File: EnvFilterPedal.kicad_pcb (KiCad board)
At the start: 4 copper layers, 80 x 52 mm, 114 parts, among them J101 ScopeGroundLoop, J102 IO, Q101 BC857, Q102 BC857, Q103 BC847, U101 TL074, U102 TL074, U103 TL074, U104 LM13700, U105 AZ34063U

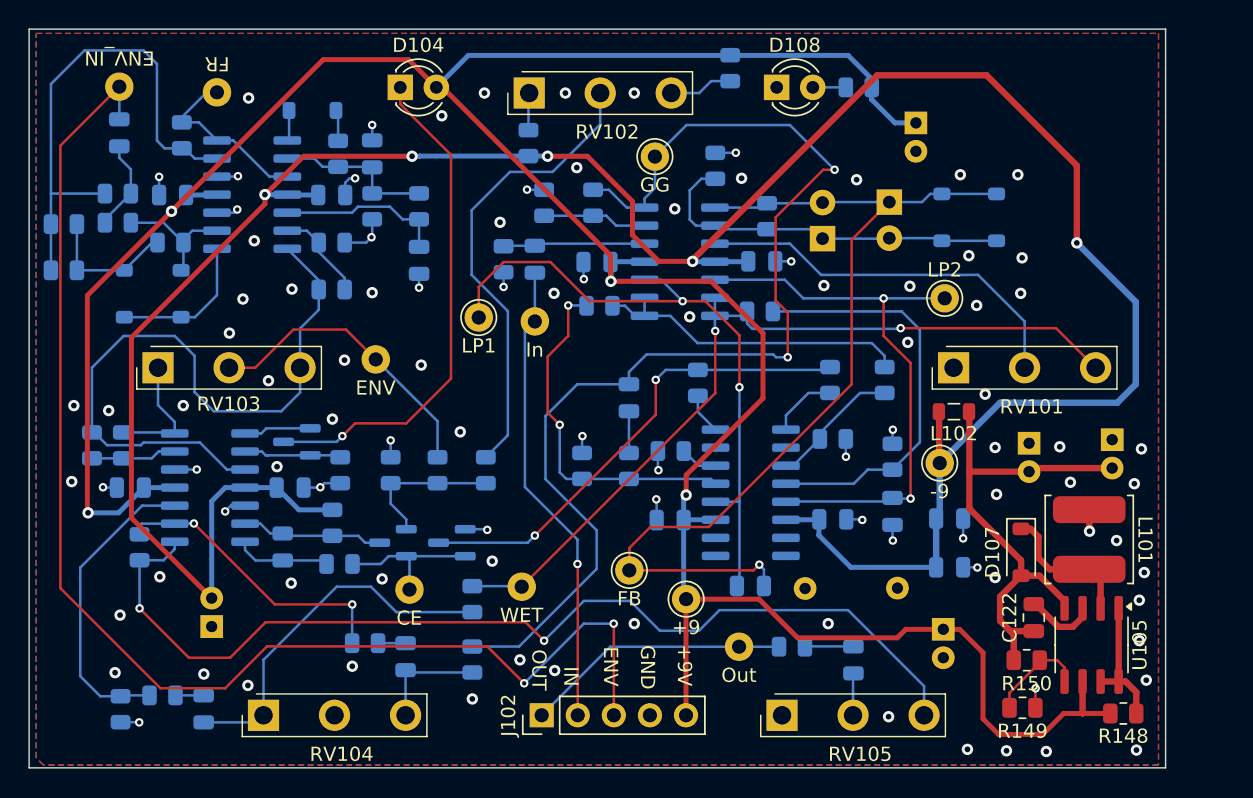
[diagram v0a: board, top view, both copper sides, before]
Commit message: new layout
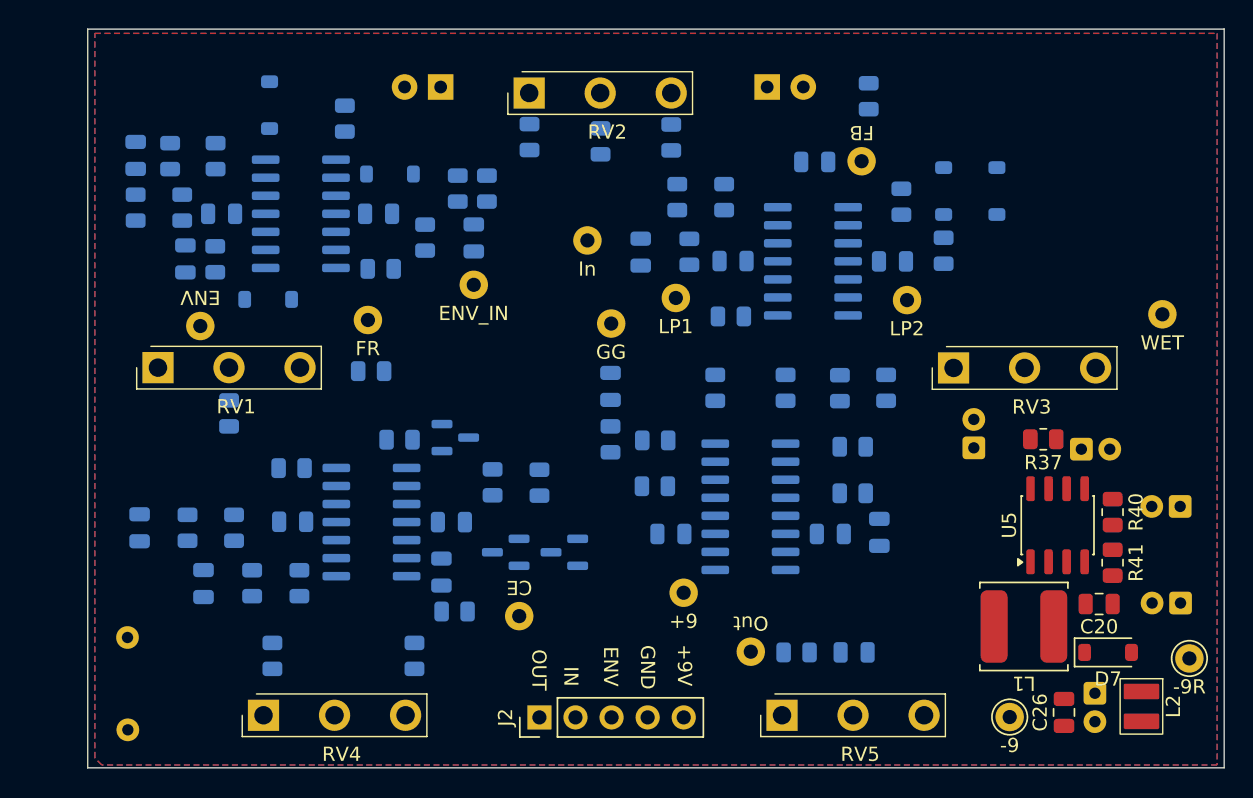
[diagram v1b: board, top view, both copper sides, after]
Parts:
- removed C101, C102, C103, C106, C108, C111, C112, C114, C115, C126: 100n, Capacitor_SMD:C_0805_2012Metric
- removed C104, C109, C113, C118, C119, C120, C125: 1u, Capacitor_SMD:C_0805_2012Metric
- removed C105: 220u, Capacitor_THT:CP_Radial_D5.0mm_P2.00mm
- removed C107: 4n7, Capacitor_SMD:C_0805_2012Metric
- removed C110: 33n, Capacitor_SMD:C_0805_2012Metric
- removed C116, C117: 1n, Capacitor_SMD:C_0805_2012Metric
- removed C121: 100u, Capacitor_THT:CP_Radial_D5.0mm_P2.00mm
- removed C122: 470p, Capacitor_SMD:C_0805_2012Metric
- removed C123, C124: 470u, Capacitor_THT:CP_Radial_D5.0mm_P2.00mm
- removed D101, D102, D103, D109, D110: 1N4148W, Diode_SMD:D_SOD-123
- removed D104, D105, D106, D108: LED, LED_THT:LED_D3.0mm
- removed D107: PMEG3030, Diode_SMD:D_SOD-123
- removed J101: ScopeGroundLoop, Connector:THT_GND_WIRE
- removed J102: IO, Connector_PinHeader_2.54mm:PinHeader_1x05_P2.54mm_Vertical
- removed L101: 68uH, Inductor_SMD:L_TDK_VLS6045EX_VLS6045AF
- removed L102: 1u, Inductor_SMD:L_0805_2012Metric
- removed Q101, Q102: BC857, Package_TO_SOT_SMD:SOT-23
- removed Q103: BC847, Package_TO_SOT_SMD:SOT-23
- removed R101, R102, R103, R104, R105, R108, R112, R113, R117, R118, R120, R124: 100k, Resistor_SMD:R_0805_2012Metric
- removed R106, R125, R126, R129, R130: 1k, Resistor_SMD:R_0805_2012Metric
- removed R107: 22k, Resistor_SMD:R_0805_2012Metric
- removed R109: 5k1, Resistor_SMD:R_0805_2012Metric
- removed R110, R136: 6k8, Resistor_SMD:R_0805_2012Metric
- removed R111, R135: 10k, Resistor_SMD:R_0805_2012Metric
- removed R114, R119: 2k2, Resistor_SMD:R_0805_2012Metric
- removed R115, R137, R139: 470k, Resistor_SMD:R_0805_2012Metric
- removed R116, R133, R134: 4k7, Resistor_SMD:R_0805_2012Metric
- removed R121: 1M, Resistor_SMD:R_0805_2012Metric
- removed R122, R141, R142: 47k, Resistor_SMD:R_0805_2012Metric
- removed R123, R154: 12k, Resistor_SMD:R_0805_2012Metric
- removed R127, R128, R131, R132: 33k, Resistor_SMD:R_0805_2012Metric
- removed R138, R140: 1Meg, Resistor_SMD:R_0805_2012Metric
- removed R143: 220, Resistor_SMD:R_0805_2012Metric
- removed R148: 0.24R, Resistor_SMD:R_0805_2012Metric
- removed R149: 51k, Resistor_SMD:R_0805_2012Metric
- removed R150: 8k2, Resistor_SMD:R_0805_2012Metric
- removed RV101, RV104: 100kB, Potentiometer_THT:Potentiometer_Alpha_RV16AF_42_VeryLong
- removed RV102, RV103: 10kB, Potentiometer_THT:Potentiometer_Alpha_RV16AF_42_VeryLong
- removed RV105: 100kA, Potentiometer_THT:Potentiometer_Alpha_RV16AF_42_VeryLong
- removed TP101: In, TestPoint:TestPoint_THTPad_D2.0mm_Drill1.0mm_VAL
- removed TP102: Out, TestPoint:TestPoint_THTPad_D2.0mm_Drill1.0mm_VAL
- removed TP103: CE, TestPoint:TestPoint_THTPad_D2.0mm_Drill1.0mm_VAL
- removed TP104: WET, TestPoint:TestPoint_THTPad_D2.0mm_Drill1.0mm_VAL
- removed TP105: ENV, TestPoint:TestPoint_THTPad_D2.0mm_Drill1.0mm_VAL
- removed TP106: ENV_IN, TestPoint:TestPoint_THTPad_D2.0mm_Drill1.0mm_VAL
- removed TP107: GG, TestPoint:TestPoint_THTPad_D2.0mm_Drill1.0mm_VAL
- removed TP108: FR, TestPoint:TestPoint_THTPad_D2.0mm_Drill1.0mm_VAL
- removed TP109: +9, TestPoint:TestPoint_THTPad_D2.0mm_Drill1.0mm_VAL
- removed TP110: -9, TestPoint:TestPoint_THTPad_D2.0mm_Drill1.0mm_VAL
- removed TP111: LP1, TestPoint:TestPoint_THTPad_D2.0mm_Drill1.0mm_VAL
- removed TP112: LP2, TestPoint:TestPoint_THTPad_D2.0mm_Drill1.0mm_VAL
- removed TP113: FB, TestPoint:TestPoint_THTPad_D2.0mm_Drill1.0mm_VAL
- removed U101, U102, U103: TL074, Package_SO:SOIC-14_3.9x8.7mm_P1.27mm
- removed U104: LM13700, Package_SO:SOIC-16_3.9x9.9mm_P1.27mm
- removed U105: AZ34063U, Package_SO:SO-8_3.9x4.9mm_P1.27mm
- added C10: 100n, Capacitor_SMD:C_0805_2012Metric, B.Cu at (60.4, 80.2)
- added C11: 1u, Capacitor_SMD:C_0805_2012Metric, B.Cu at (15.0, 60.9)
- added C12: 1u, Capacitor_SMD:C_0805_2012Metric, B.Cu at (44.9, 69.8)
- added C13: 33n, Capacitor_SMD:C_0805_2012Metric, B.Cu at (11.5, 53.6)
- added C14: 1n, Capacitor_SMD:C_0805_2012Metric, B.Cu at (59.3, 54.0)
- added C15: 1n, Capacitor_SMD:C_0805_2012Metric, B.Cu at (63.9, 80.1)
- added C16: 4n7, Capacitor_SMD:C_0805_2012Metric, B.Cu at (33.0, 82.9)
- added C17: 220u, Capacitor_THT:CP_Radial_D5.0mm_P2.00mm, B.Cu at (78.1, 74.3)
- added C18: 1u, Capacitor_SMD:C_0805_2012Metric, B.Cu at (16.3, 83.7)
- added C19: 1u, Capacitor_SMD:C_0805_2012Metric, B.Cu at (11.8, 79.8)
- added C2: 100n, Capacitor_SMD:C_0805_2012Metric, B.Cu at (17.6, 57.7)
- added C20: 470p, Capacitor_SMD:C_0805_2012Metric, F.Cu at (79.3, 85.2)
- added C21: 220u, Capacitor_THT:CP_Radial_D5.0mm_P2.00mm, B.Cu at (85.1, 85.1)
- added C22: 470u, Capacitor_THT:CP_Radial_D5.0mm_P2.00mm, B.Cu at (85.0, 78.3)
- added C23: 1u, Capacitor_SMD:C_0805_2012Metric, B.Cu at (62.1, 88.6)
- added C24: 220u, Capacitor_THT:CP_Radial_D5.0mm_P2.00mm, B.Cu at (79.0, 91.4)
- added C25: 100u, Capacitor_THT:CP_Radial_D5.0mm_P2.00mm, B.Cu at (70.5, 74.2)
- added C26: 10u, Capacitor_SMD:C_0805_2012Metric, F.Cu at (76.8, 92.8)
- added C3: 100n, Capacitor_SMD:C_0805_2012Metric, B.Cu at (22.6, 79.4)
- added C4: 100n, Capacitor_SMD:C_0805_2012Metric, B.Cu at (33.7, 79.4)
- added C5: 100n, Capacitor_SMD:C_0805_2012Metric, B.Cu at (35.3, 59.4)
- added C6: 1u, Capacitor_SMD:C_0805_2012Metric, B.Cu at (47.0, 60.4)
- added C7: 100n, Capacitor_SMD:C_0805_2012Metric, B.Cu at (53.5, 61.0)
- added C8: 100n, Capacitor_SMD:C_0805_2012Metric, B.Cu at (64.8, 61.0)
- added C9: 100n, Capacitor_SMD:C_0805_2012Metric, B.Cu at (49.2, 80.2)
- added D1: 1N4148W, Diode_SMD:D_SOD-123, B.Cu at (29.4, 54.9)
- added D2: 1N4148W, Diode_SMD:D_SOD-123, B.Cu at (20.9, 50.0)
- added D3: 1N4148W, Diode_SMD:D_SOD-123, B.Cu at (20.8, 63.7)
- added D4: 1N4148W, Diode_SMD:D_SOD-123, B.Cu at (68.4, 56.1)
- added D5: 1N4148W, Diode_SMD:D_SOD-123, B.Cu at (72.1, 56.1)
- added D6: LED, LED_THT:LED_D3.0mm, B.Cu at (33.0, 48.8)
- added D7: PMEG3030, Diode_SMD:D_SOD-123, F.Cu at (80.0, 88.6)
- added D8: LED, LED_THT:LED_D3.0mm, B.Cu at (56.0, 48.8)
- added J1: ScopeGroundLoop, Connector_Pin:THT_GND_WIRE, B.Cu at (10.9, 90.6)
- added J2: IO, Connector_PinHeader_2.54mm:PinHeader_1x05_P2.54mm_Vertical, F.Cu at (39.9, 93.2)
- added L1: 68uH, Inductor_SMD:L_TDK_VLS6045EX_VLS6045AF, F.Cu at (74.0, 86.8)
- added L2: 4u7, Inductor_SMD:L_Bourns_SRP3212, F.Cu at (82.3, 92.4)
- added Q1: BC847, Package_TO_SOT_SMD:SOT-23, B.Cu at (34.0, 73.5)
- added Q2: BC857, Package_TO_SOT_SMD:SOT-23, B.Cu at (37.5, 81.5)
- added Q3: BC857, Package_TO_SOT_SMD:SOT-23, B.Cu at (41.7, 81.5)
- added R1: 100k, Resistor_SMD:R_0805_2012Metric, B.Cu at (36.2, 55.9)
- added R10: 47k, Resistor_SMD:R_0805_2012Metric, B.Cu at (34.2, 55.9)
- added R11: 100k, Resistor_SMD:R_0805_2012Metric, B.Cu at (31.9, 59.4)
- added R12: 22k, Resistor_SMD:R_0805_2012Metric, B.Cu at (14.8, 57.3)
- added R13: 33k, Resistor_SMD:R_0805_2012Metric, B.Cu at (44.9, 73.6)
- added R14: 100k, Resistor_SMD:R_0805_2012Metric, B.Cu at (28.8, 61.6)
- added R15: 1k, Resistor_SMD:R_0805_2012Metric, B.Cu at (48.0, 76.9)
- added R16: 100k, Resistor_SMD:R_0805_2012Metric, B.Cu at (11.5, 57.3)
- added R17: 1k, Resistor_SMD:R_0805_2012Metric, B.Cu at (48.1, 73.7)
- added R18: 33k, Resistor_SMD:R_0805_2012Metric, B.Cu at (53.4, 64.9)
- added R19: 4k7, Resistor_SMD:R_0805_2012Metric, B.Cu at (52.3, 70.0)
- added R2: 1M, Resistor_SMD:R_0805_2012Metric, B.Cu at (50.5, 60.4)
- added R20: 5k1, Resistor_SMD:R_0805_2012Metric, B.Cu at (13.9, 53.6)
- added R21: 100k, Resistor_SMD:R_0805_2012Metric, B.Cu at (17.1, 53.6)
- added R22: 10k, Resistor_SMD:R_0805_2012Metric, B.Cu at (65.4, 56.9)
- added R23: 33k, Resistor_SMD:R_0805_2012Metric, B.Cu at (61.1, 70.0)
- added R24: 1k, Resistor_SMD:R_0805_2012Metric, B.Cu at (62.0, 77.4)
- added R25: 2k2, Resistor_SMD:R_0805_2012Metric, B.Cu at (30.1, 73.6)
- added R26: 6k8, Resistor_SMD:R_0805_2012Metric, B.Cu at (68.4, 60.3)
- added R27: 1k, Resistor_SMD:R_0805_2012Metric, B.Cu at (62.0, 74.1)
- added R28: 33k, Resistor_SMD:R_0805_2012Metric, B.Cu at (64.3, 70.0)
- added R29: 4k7, Resistor_SMD:R_0805_2012Metric, B.Cu at (57.2, 70.0)
- added R3: 100k, Resistor_SMD:R_0805_2012Metric, B.Cu at (28.1, 68.8)
- added R30: 6k8, Resistor_SMD:R_0805_2012Metric, B.Cu at (49.2, 52.3)
- added R31: 10k, Resistor_SMD:R_0805_2012Metric, B.Cu at (39.2, 52.3)
- added R32: 100k, Resistor_SMD:R_0805_2012Metric, B.Cu at (18.1, 71.8)
- added R33: 100k, Resistor_SMD:R_0805_2012Metric, B.Cu at (44.2, 52.6)
- added R34: 2k2, Resistor_SMD:R_0805_2012Metric, B.Cu at (39.9, 76.6)
- added R35: 470k, Resistor_SMD:R_0805_2012Metric, B.Cu at (36.6, 76.6)
- added R36: 4k7, Resistor_SMD:R_0805_2012Metric, B.Cu at (34.0, 85.7)
- added R37: 0.24R, Resistor_SMD:R_0805_2012Metric, F.Cu at (75.4, 73.6)
- added R38: 47k, Resistor_SMD:R_0805_2012Metric, B.Cu at (21.1, 88.8)
- added R39: 47k, Resistor_SMD:R_0805_2012Metric, B.Cu at (31.1, 88.8)
- added R4: 12k, Resistor_SMD:R_0805_2012Metric, B.Cu at (49.6, 56.5)
- added R40: 51k, Resistor_SMD:R_0805_2012Metric, F.Cu at (80.3, 78.7)
- added R41: 8k2, Resistor_SMD:R_0805_2012Metric, F.Cu at (80.3, 82.3)
- added R42: 470k, Resistor_SMD:R_0805_2012Metric, B.Cu at (19.7, 83.7)
- added R43: 470k, Resistor_SMD:R_0805_2012Metric, B.Cu at (15.2, 79.8)
- added R44: 1Meg, Resistor_SMD:R_0805_2012Metric, B.Cu at (18.4, 79.8)
- added R45: 1Meg, Resistor_SMD:R_0805_2012Metric, B.Cu at (23.0, 83.7)
- added R46: 220, Resistor_SMD:R_0805_2012Metric, B.Cu at (58.0, 88.6)
- added R47: 12k, Resistor_SMD:R_0805_2012Metric, B.Cu at (63.1, 49.4)
- added R5: 100k, Resistor_SMD:R_0805_2012Metric, B.Cu at (26.2, 51.0)
- added R6: 47k, Resistor_SMD:R_0805_2012Metric, B.Cu at (52.9, 56.5)
- added R7: 100k, Resistor_SMD:R_0805_2012Metric, B.Cu at (22.5, 75.6)
- added R8: 1k, Resistor_SMD:R_0805_2012Metric, B.Cu at (17.1, 60.9)
- added RV1: 10kB, Potentiometer_THT:Potentiometer_Alpha_RV16AF_42_Single_Long, F.Cu at (13.1, 68.5)
- added RV2: 10kB, Potentiometer_THT:Potentiometer_Alpha_RV16AF_42_Single_Long, F.Cu at (39.2, 49.2)
- added RV3: 100kB, Potentiometer_THT:Potentiometer_Alpha_RV16AF_42_Single_Long, F.Cu at (69.1, 68.5)
- added RV4: 100kB, Potentiometer_THT:Potentiometer_Alpha_RV16AF_42_Single_Long, F.Cu at (20.5, 93.0)
- added RV5: 100kA, Potentiometer_THT:Potentiometer_Alpha_RV16AF_42_Single_Long, F.Cu at (57.0, 93.0)
- added TP1: LP1, TestPoint:TestPoint_THTPad_D2.0mm_Drill1.0mm_VAL, B.Cu at (49.5, 63.6)
- added TP10: ENV, TestPoint:TestPoint_THTPad_D2.0mm_Drill1.0mm_VAL, B.Cu at (16.1, 65.6)
- added TP11: ENV_IN, TestPoint:TestPoint_THTPad_D2.0mm_Drill1.0mm_VAL, B.Cu at (35.3, 62.7)
- added TP12: +9, TestPoint:TestPoint_THTPad_D2.0mm_Drill1.0mm_VAL, B.Cu at (50.1, 84.4)
- added TP13: -9, TestPoint:TestPoint_THTPad_D2.0mm_Drill1.0mm_VAL, F.Cu at (73.0, 93.1)
- added TP14: -9R, TestPoint:TestPoint_THTPad_D2.0mm_Drill1.0mm_VAL, F.Cu at (85.7, 89.0)
- added TP2: In, TestPoint:TestPoint_THTPad_D2.0mm_Drill1.0mm_VAL, B.Cu at (43.3, 59.6)
- added TP3: LP2, TestPoint:TestPoint_THTPad_D2.0mm_Drill1.0mm_VAL, B.Cu at (65.8, 63.8)
- added TP4: Out, TestPoint:TestPoint_THTPad_D2.0mm_Drill1.0mm_VAL, B.Cu at (54.8, 88.5)
- added TP5: FR, TestPoint:TestPoint_THTPad_D2.0mm_Drill1.0mm_VAL, B.Cu at (27.9, 65.2)
- added TP6: GG, TestPoint:TestPoint_THTPad_D2.0mm_Drill1.0mm_VAL, B.Cu at (45.0, 65.4)
- added TP7: FB, TestPoint:TestPoint_THTPad_D2.0mm_Drill1.0mm_VAL, B.Cu at (62.6, 54.0)
- added TP8: CE, TestPoint:TestPoint_THTPad_D2.0mm_Drill1.0mm_VAL, B.Cu at (38.5, 86.0)
- added TP9: WET, TestPoint:TestPoint_THTPad_D2.0mm_Drill1.0mm_VAL, B.Cu at (83.8, 64.8)
- added U1: TL074, Package_SO:SOIC-14_3.9x8.7mm_P1.27mm, B.Cu at (23.1, 57.7)
- added U2: TL074, Package_SO:SOIC-14_3.9x8.7mm_P1.27mm, B.Cu at (28.1, 79.4)
- added U3: TL074, Package_SO:SOIC-14_3.9x8.7mm_P1.27mm, B.Cu at (59.2, 61.0)
- added U4: LM13700, Package_SO:SOIC-16_3.9x9.9mm_P1.27mm, B.Cu at (54.8, 78.3)
- added U5: AZ34063U, Package_SO:SO-8_3.9x4.9mm_P1.27mm, F.Cu at (76.4, 79.6)
- C1: value 220u -> 100n; footprint Capacitor_THT:CP_Radial_D5.0mm_P2.00mm -> Capacitor_SMD:C_0805_2012Metric
- moved C1 49.4 mm to (28.6, 57.7), turned to 0 degrees
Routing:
- net +9V: track 202.6 -> 0.00 mm, vias 4 -> 0
- net -9V: track 187.0 -> 0.00 mm, vias 5 -> 0
- net ENV_IN: track 91.7 -> 0.00 mm, vias 2 -> 0
- net /GTR_GAIN: track 81.3 -> 0.00 mm, vias 2 -> 0
- net Net-(R140-Pad2): track 71.8 -> 0.00 mm, vias 2 -> 0
- net /Feedback: track 67.1 -> 0.00 mm, vias 1 -> 0
- net /WET: track 58.6 -> 0.00 mm, vias 2 -> 0
- net /EnvPos: track 47.3 -> 0.00 mm
- net /LP1: track 46.1 -> 0.00 mm, vias 2 -> 0
- net GND: track 42.2 -> 0.00 mm, vias 98 -> 0
- net /LP2: track 40.5 -> 0.00 mm, vias 2 -> 0
- net /-9RAW: track 36.3 -> 0.00 mm
- net Net-(U101B--): track 35.9 -> 0.00 mm
- net Net-(D104-K): track 35.6 -> 0.00 mm, vias 1 -> 0
- net Iabc: track 34.1 -> 0.00 mm, vias 2 -> 0
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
